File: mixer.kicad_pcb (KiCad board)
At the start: 2 copper layers, 86.4 x 119.4 mm, 35 parts, among them J1 in1, J10 PowDistr, J11 12v, J2 in2, J3 in3, J4 power, J5 interface1, J6 interface2, J7 interface3, J8 PowDistr, J9 PowDistr, U1 NE5532

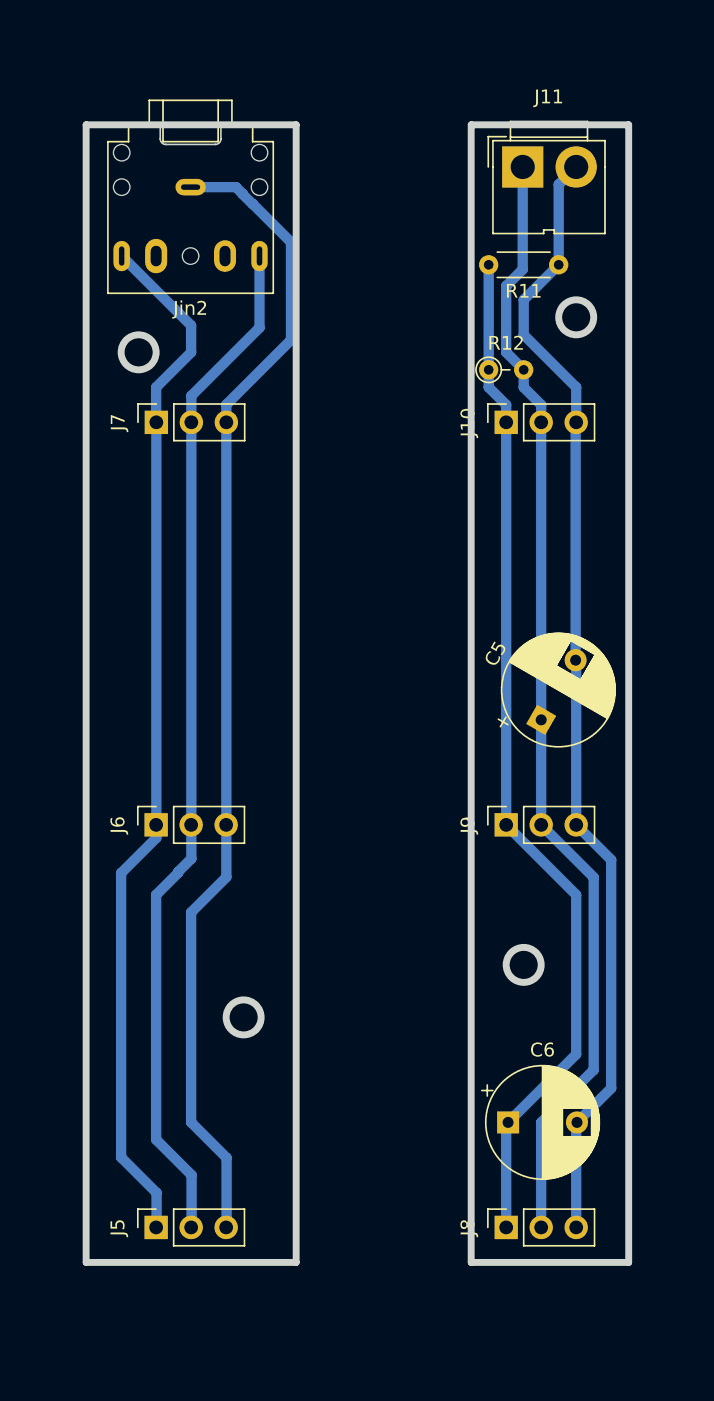
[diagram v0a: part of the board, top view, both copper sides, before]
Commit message: add box
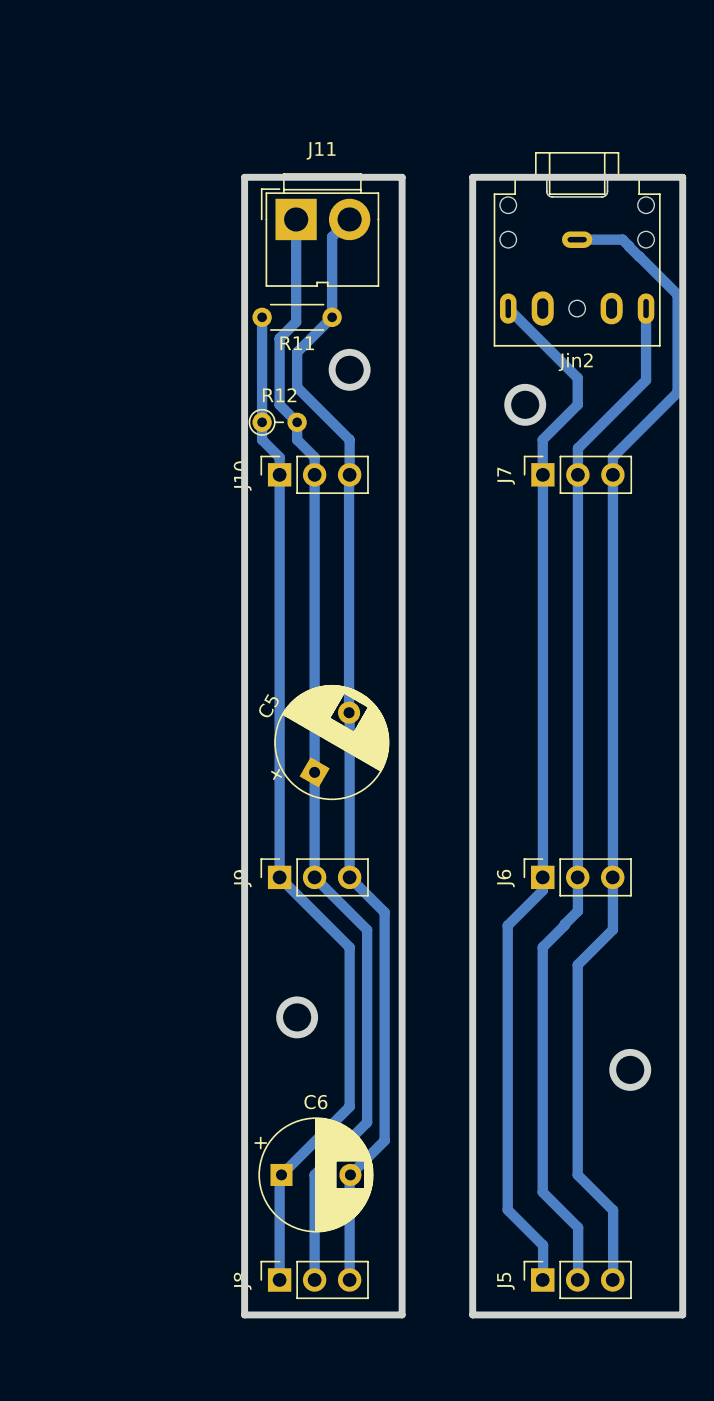
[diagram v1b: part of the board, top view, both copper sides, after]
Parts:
- moved J6 28.3 mm to (110.7, 100.9)
- moved J7 28.3 mm to (110.7, 71.7)
- moved Jin2 28.3 mm to (113.2, 54.6)
- moved J5 28.3 mm to (110.7, 130.1)
- moved C5 16.9 mm to (94.1, 93.2)
- moved C6 16.9 mm to (91.7, 122.5)
- moved J10 16.9 mm to (91.6, 71.7)
- moved J11 16.9 mm to (92.8, 53.1)
- moved J9 16.9 mm to (91.6, 100.9)
- moved R11 16.9 mm to (95.4, 60.2)
- moved R12 16.9 mm to (90.3, 67.8)
- moved J8 16.9 mm to (91.6, 130.1)
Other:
- board size 86.4 x 119.4 mm -> 90.3 x 119.4 mm

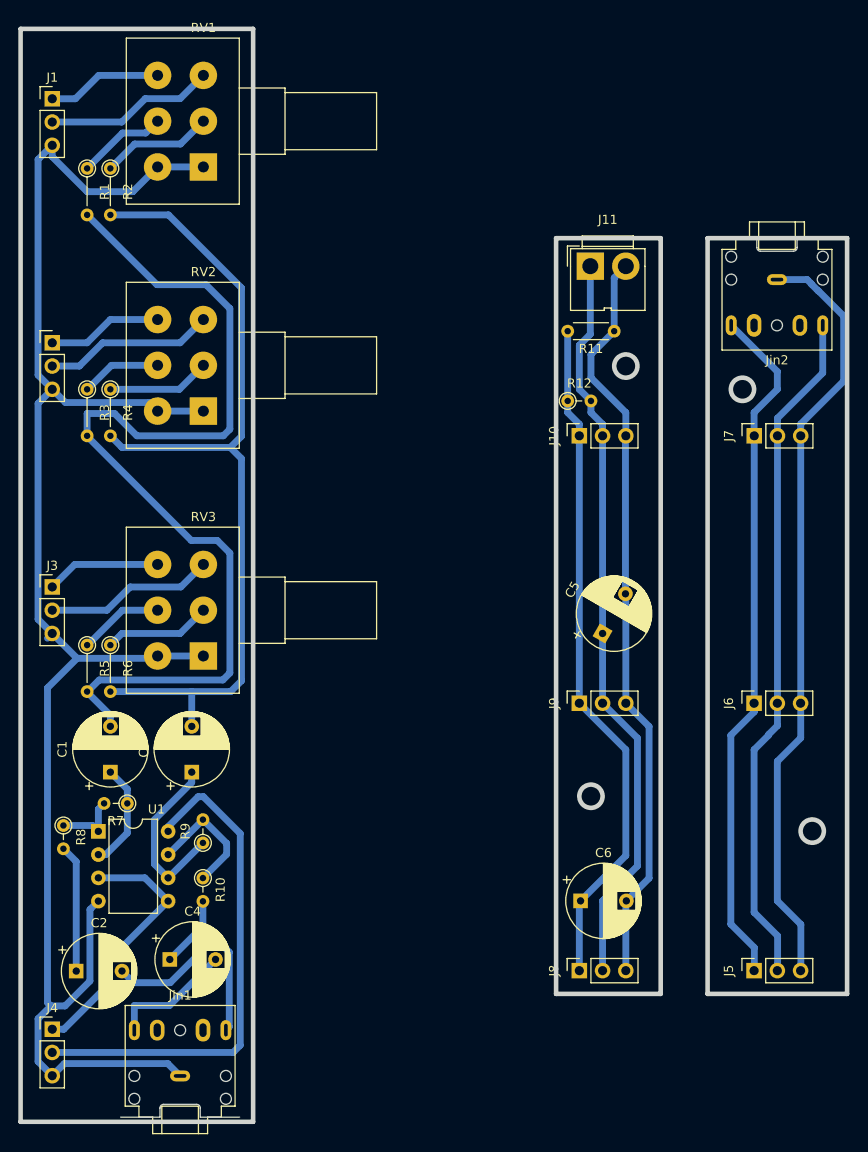
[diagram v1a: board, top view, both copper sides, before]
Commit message: update box
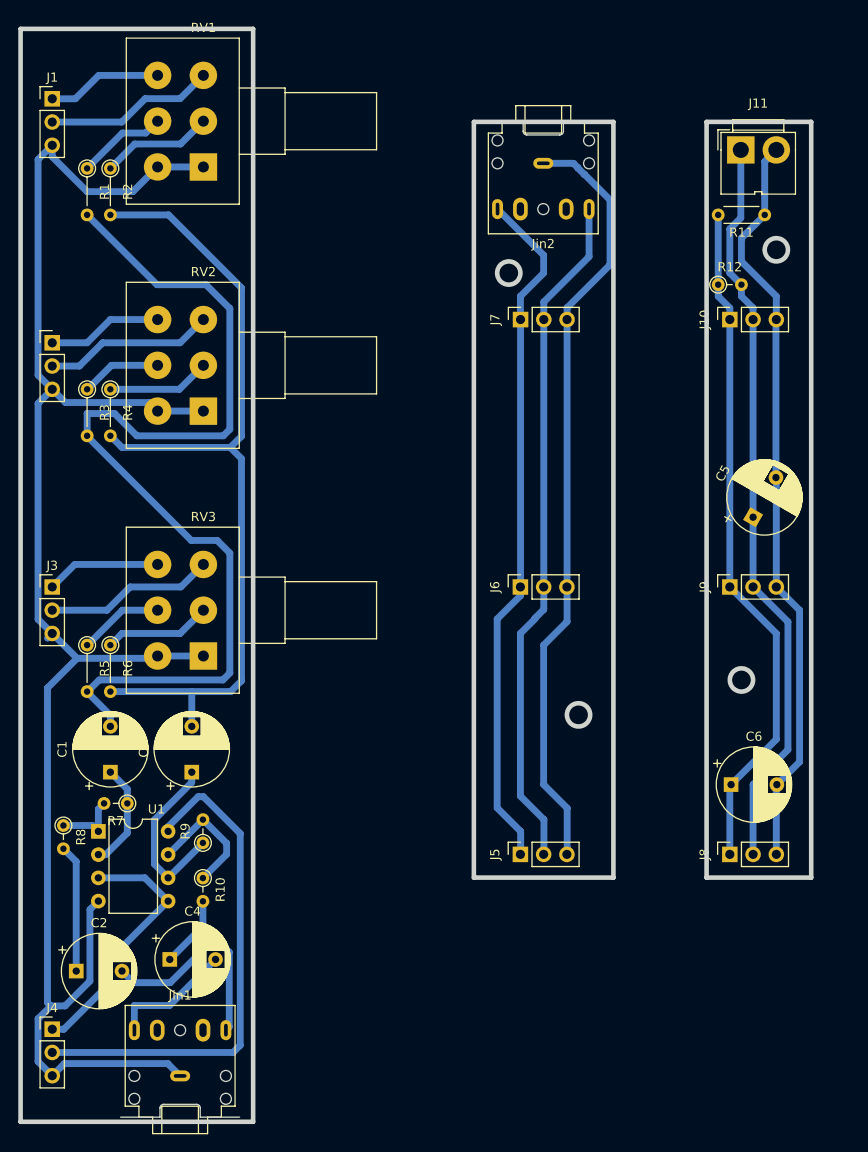
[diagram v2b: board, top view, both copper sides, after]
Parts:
- moved J5 28.5 mm to (85.1, 117.4)
- moved J6 28.5 mm to (85.1, 88.2)
- moved J7 28.5 mm to (85.1, 59.0)
- moved Jin2 28.5 mm to (87.6, 41.9)
- moved C5 20.8 mm to (110.5, 80.5)
- moved C6 20.8 mm to (108.1, 109.8)
- moved J10 20.8 mm to (108.0, 59.0)
- moved J9 20.8 mm to (108.0, 88.2)
- moved R12 20.8 mm to (106.7, 55.1)
- moved J11 20.8 mm to (109.2, 40.4)
- moved R11 20.8 mm to (111.8, 47.5)
- moved J8 20.8 mm to (108.0, 117.4)
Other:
- board size 90.3 x 119.4 mm -> 86.4 x 119.4 mm
